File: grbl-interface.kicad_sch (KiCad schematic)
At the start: 12 parts, among them U6 USBLC6-2SC6, U7 ADUM4160, U8 ATmega16U2-A, U9 ATmega328P-A, Y1 Crystal_GND24

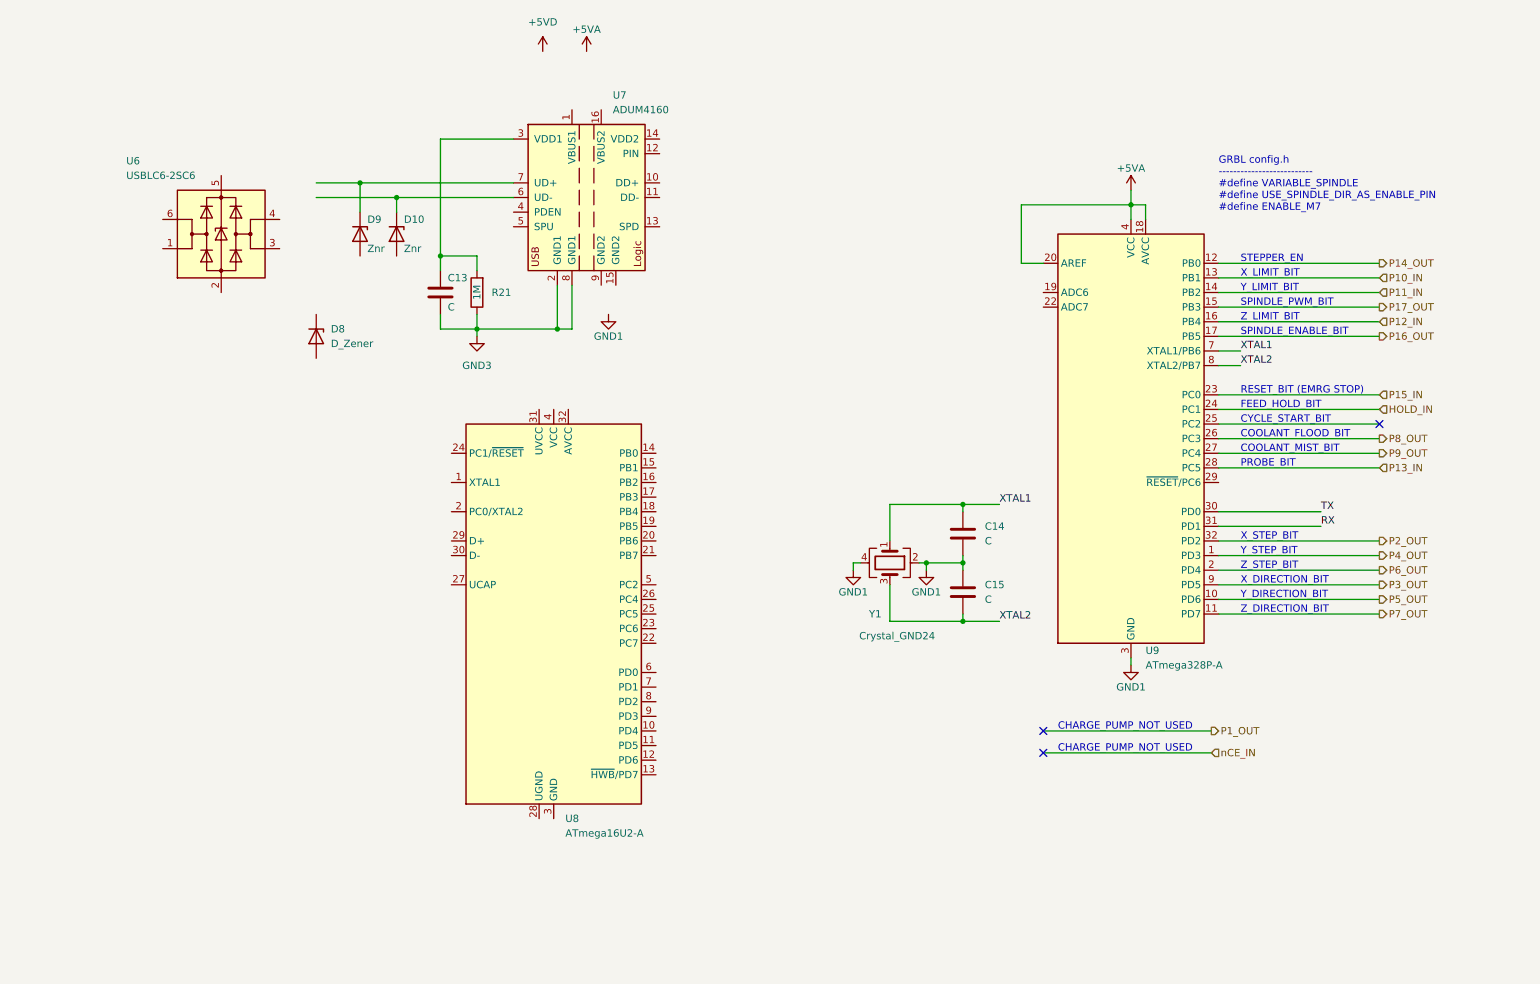
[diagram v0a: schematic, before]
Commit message: GRBL PCB controller work
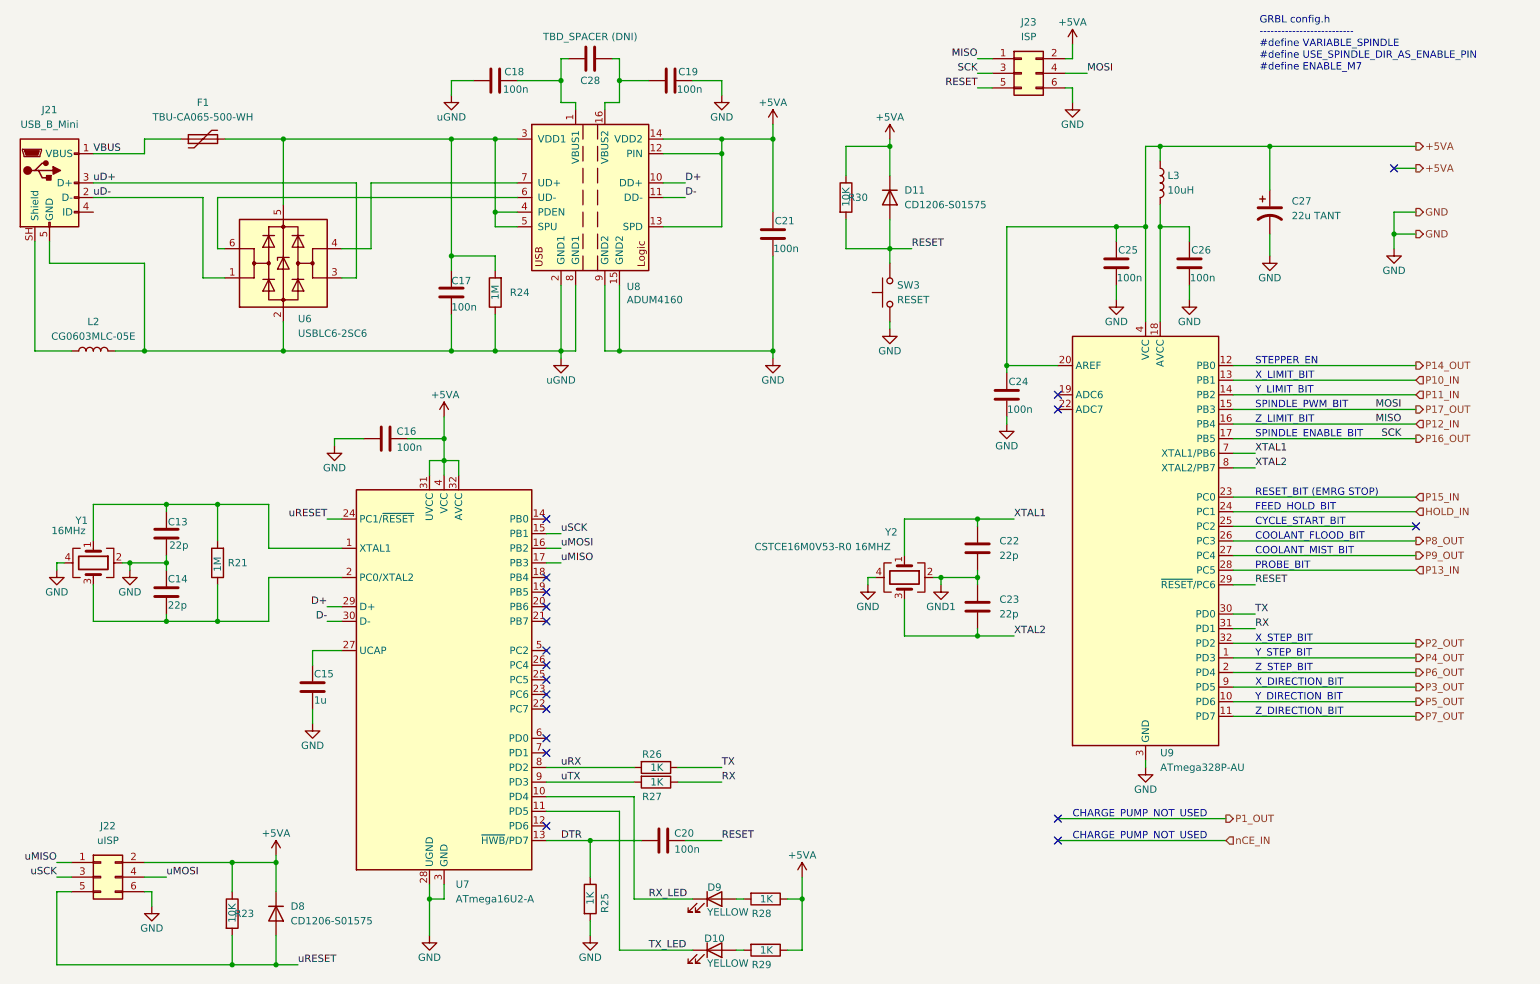
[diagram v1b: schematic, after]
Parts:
- removed D10, D9: Znr, symbol Device:D_Zener
- removed D8: D_Zener, symbol Device:D_Zener
- added C13, C14: 22p, Capacitor_SMD:C_0402_1005Metric_Pad0.74x0.62mm_HandSolder, symbol Device:C
- added C15: 1u, Capacitor_SMD:C_0603_1608Metric, symbol Device:C
- added C16, C18, C19, C20, C21, C24, C25, C26: 100n, Capacitor_SMD:C_0603_1608Metric, symbol Device:C
- added C27: 22u TANT, Capacitor_SMD:C_1206_3216Metric, symbol Device:C_Polarized_US
- added C28: TBD_SPACER (DNI), symbol Device:C
- added D10, D9: YELLOW, -Project:LED_0402_DOT, symbol Device:LED
- added D11, D8: CD1206-S01575, -Project:D_SOD-523_DOT, symbol Device:D
- added F1: TBU-CA065-500-WH, Fuse:Fuse_Bourns_TBU-CA, symbol Power_Protection:TBU-CA065-500-WH
- added J21: USB_B_Mini, Connector_USB:USB_Mini-B_Wuerth_65100516121_Horizontal, symbol Connector:USB_B_Mini
- added J22: uISP, -Project:ISP_SMD_100mil, symbol Connector_Generic:Conn_02x03_Odd_Even
- added J23: ISP, -Project:ISP_SMD_100mil, symbol Connector_Generic:Conn_02x03_Odd_Even
- added L2: CG0603MLC-05E, symbol Device:L
- added L3: 10uH, symbol Device:L
- added R21: 1M, symbol Device:R
- added R23, R30: 10K, symbol Device:R
- added R25, R26, R27, R28, R29: 1K, symbol Device:R
- added SW3: RESET, symbol Switch:SW_Push
- added Y1: 16MHz, symbol Device:Crystal_GND24
- C17: renamed from C13; value C -> 100n; footprint (none) -> Capacitor_SMD:C_0603_1608Metric
- C22: renamed from C14; value C -> 22p; footprint (none) -> Capacitor_SMD:C_0402_1005Metric_Pad0.74x0.62mm_HandSolder
- C23: renamed from C15; value C -> 22p; footprint (none) -> Capacitor_SMD:C_0402_1005Metric_Pad0.74x0.62mm_HandSolder
- U9: value ATmega328P-A -> ATmega328P-AU
- Y2: renamed from Y1; value Crystal_GND24 -> CSTCE16M0V53-R0 16MHZ
- renumbered R21 to R24, U8 to U7, U7 to U8
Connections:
- net GND3 is gone; now on net uGND: C17.2, R24.1, U8.2 (GND1), U8.8 (GND1)
- net +5VA: now also U7.31 (UVCC), U7.32 (AVCC), U7.4 (VCC), U8.12 (PIN), U8.13 (SPD), U8.14 (VDD2), C16.2, C21.2, C24.2, C25.2, C27.1, D11.1 (K), D8.1 (K), J22.2 (Pin_2), J23.2 (Pin_2), L3.1, R23.1, R28.1, R29.1, R30.1; no longer U9.18 (AVCC)
- net GND1: no longer U9.21 (GND), U9.3 (GND), U9.5 (GND), Y2.4
- net P12_IN: now also J23.1 (Pin_1)
- net P16_OUT: now also J23.3 (Pin_3)
- net P17_OUT: now also J23.4 (Pin_4)
- net RX: now also R27.1
- net TX: now also R26.1
- net uD-: now reaches U6.1 (I/O1)
- net uD-: now also J21.2 (D-)
- net uGND: now reaches U6.2 (GND)
- net uGND: now also C18.1, J21.5 (GND), L2.2
- net uD+: now reaches U6.3 (I/O2)
- net uD+: now also J21.3 (D+)
- net at U6.4 (I/O2): now also U8.7 (UD+)
- net at U6.5 (VBUS): now also C17.1, R24.2, U8.3 (VDD1), U8.4 (PDEN), U8.5 (SPU), F1.3
- net at U6.6 (I/O1): now also U8.6 (UD-)
- net RESET: now reaches U9.29 (~{RESET}/PC6)
- net RESET: now also C20.2, D11.2 (A), J23.5 (Pin_5), R30.2, SW3.2
- net at U7.1 (XTAL1): now also C13.1, R21.2, Y1.1
- net RX_LED: now reaches U7.10 (PD4)
- net RX_LED: now also D9.1 (K)
- net TX_LED: now reaches U7.11 (PD5)
- net TX_LED: now also D10.1 (K)
- net DTR: now reaches U7.13 (~{HWB}/PD7)
- net DTR: now also C20.1, R25.1
- net uSCK: now reaches U7.15 (PB1)
- net uSCK: now also J22.3 (Pin_3)
- net uMOSI: now reaches U7.16 (PB2)
- net uMOSI: now also J22.4 (Pin_4)
- net uMISO: now reaches U7.17 (PB3)
- net uMISO: now also J22.1 (Pin_1)
- net at U7.2 (PC0/XTAL2): now also C14.2, R21.1, Y1.3
- net uRESET: now reaches U7.24 (PC1/~{RESET})
- net uRESET: now also D8.2 (A), J22.5 (Pin_5), R23.2
- net at U7.27 (UCAP): now also C15.1
- net GND: now reaches U7.28 (UGND)
- net GND: now also U7.3 (GND), U8.15 (GND2), U8.9 (GND2), U9.21 (GND), U9.3 (GND), U9.5 (GND), Y2.4, C13.2, C14.1, C15.2, C16.1, C19.1, C21.1, C24.1, C25.1, C26.1, C27.2, J22.6 (Pin_6), J23.6 (Pin_6), R25.2, SW3.1, Y1.2, Y1.4
- net D+: now reaches U7.29 (D+)
- net D+: now also U8.10 (DD+)
- net D-: now reaches U7.30 (D-)
- net D-: now also U8.11 (DD-)
- net uRX: now reaches U7.8 (PD2)
- net uRX: now also R26.2
- net uTX: now reaches U7.9 (PD3)
- net uTX: now also R27.2
- net at U8.1 (VBUS1): now also C18.2, C28.2
- net at U8.16 (VBUS2): now also C19.2, C28.1
- new net: C26.2, L3.2, U9.18 (AVCC)
- new net: D9.2 (A), R28.2
- new net: J21.SH (Shield), L2.1
- new net: D10.2 (A), R29.2
- new net VBUS: F1.1, J21.1 (VBUS)
- no-connect marks 3 -> 19
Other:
- moved on the sheet: C17, C22, C23, R24, U6, U7, U8, U9, Y2
